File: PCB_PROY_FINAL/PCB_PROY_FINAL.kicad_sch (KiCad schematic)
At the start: 3 parts

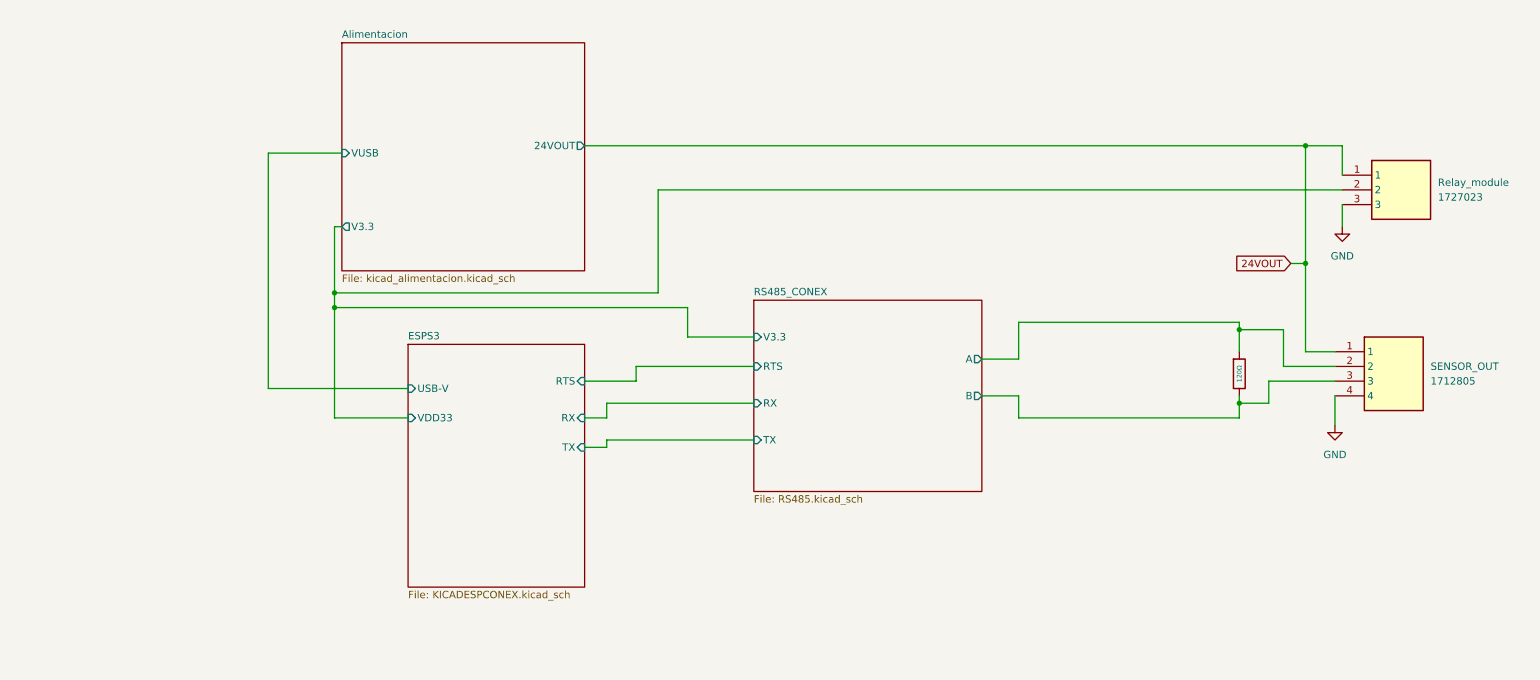
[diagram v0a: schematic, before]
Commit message: Last update pcb
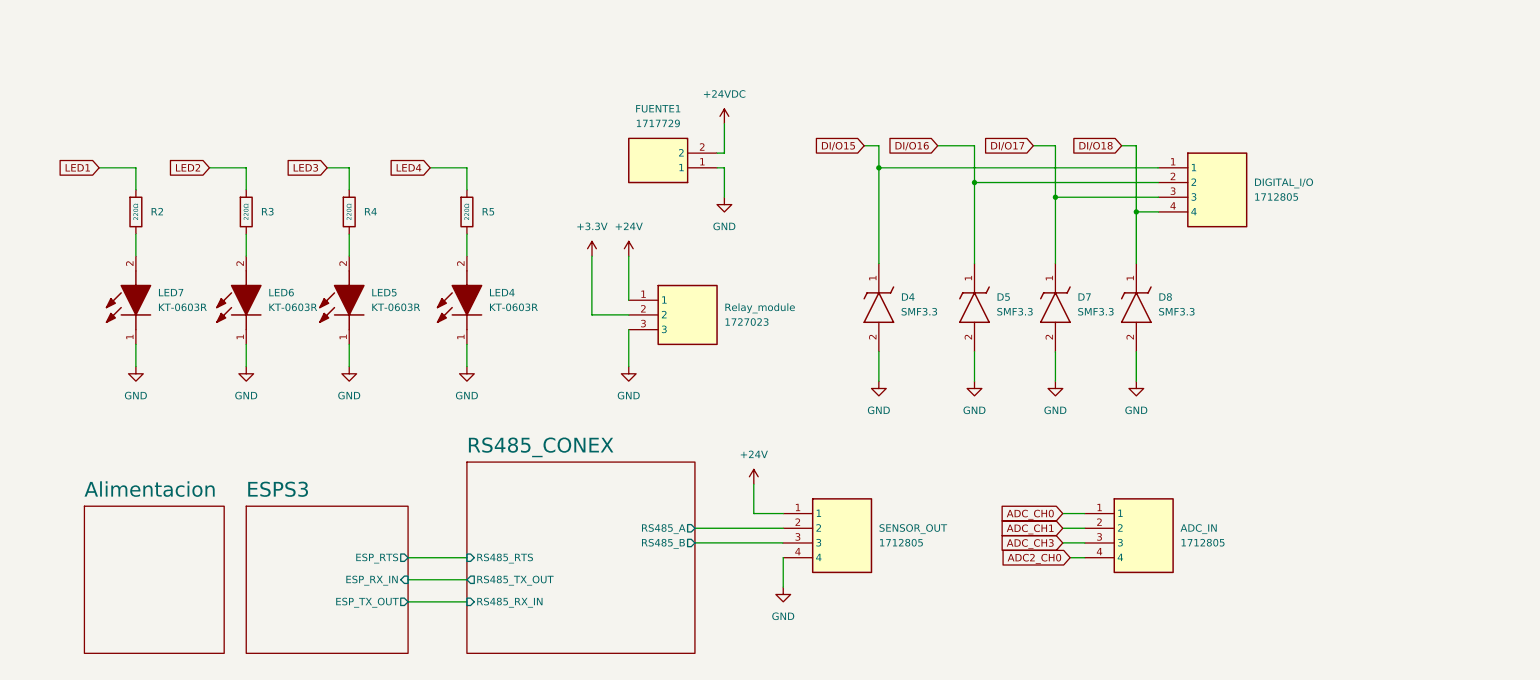
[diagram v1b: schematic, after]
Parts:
- removed R2: 120Ω, PCM_JLCPCB:R_1206, symbol PCM_JLCPCB-Resistors:1206,120Ω
- added ADC_IN, DIGITAL_I/O: 1712805, 1712805, symbol SamacSys_Parts:1712805
- added D4, D5, D7, D8: SMF3.3, SamacSys_Parts:SOD3718X108N, symbol SamacSys_Parts:SMF3.3
- added FUENTE1: 1717729, 1717729, symbol SamacSys_Parts:1717729
- added LED4, LED5, LED6, LED7: KT-0603R, LEDC1608X70N, symbol SamacSys_Parts:KT-0603R
- added R2, R3, R4, R5: 220Ω, PCM_JLCPCB:R_0603, symbol PCM_JLCPCB-Resistors:0603,220Ω
- SENSOR_OUT: JLC PART# (none) -> C90087
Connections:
- net GND: now also D4.2 (A), D5.2 (A), D7.2 (A), D8.2 (A), FUENTE1.1, LED4.1 (K), LED5.1 (K), LED6.1 (K), LED7.1 (K)
- net 24VOUT renamed +24V
- net Alimentacion/V3.3 renamed +3.3V
- net RS485_CONEX/A renamed RS485_CONEX/RS485_A
- net RS485_CONEX/B renamed RS485_CONEX/RS485_B
- new net: LED7.2 (A), R2.2
- new net: LED5.2 (A), R4.2
- new net: LED4.2 (A), R5.2
- new net: LED6.2 (A), R3.2
- new net +24VDC: FUENTE1.2
- new net ADC2_CH0: ADC_IN.4
- new net ADC_CH0: ADC_IN.1
- new net ADC_CH1: ADC_IN.2
- new net ADC_CH3: ADC_IN.3
- new net DI/O15: D4.1 (K), DIGITAL_I/O.1
- new net DI/O16: D5.1 (K), DIGITAL_I/O.2
- new net DI/O17: D7.1 (K), DIGITAL_I/O.3
- new net DI/O18: D8.1 (K), DIGITAL_I/O.4
- new net LED1: R2.1
- new net LED2: R3.1
- new net LED3: R4.1
- new net LED4: R5.1
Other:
- sheet Alimentacion ports: added none; removed 24VOUT, V3.3, VUSB
- sheet ESPS3 ports: added ESP_RTS, ESP_RX_IN, ESP_TX_OUT; removed RTS, RX, TX, USB-V, VDD33
- sheet RS485_CONEX ports: added RS485_A, RS485_B, RS485_RTS, RS485_RX_IN, RS485_TX_OUT; removed A, B, RTS, RX, TX, V3.3
- moved on the sheet: Relay_module, SENSOR_OUT

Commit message: new changes
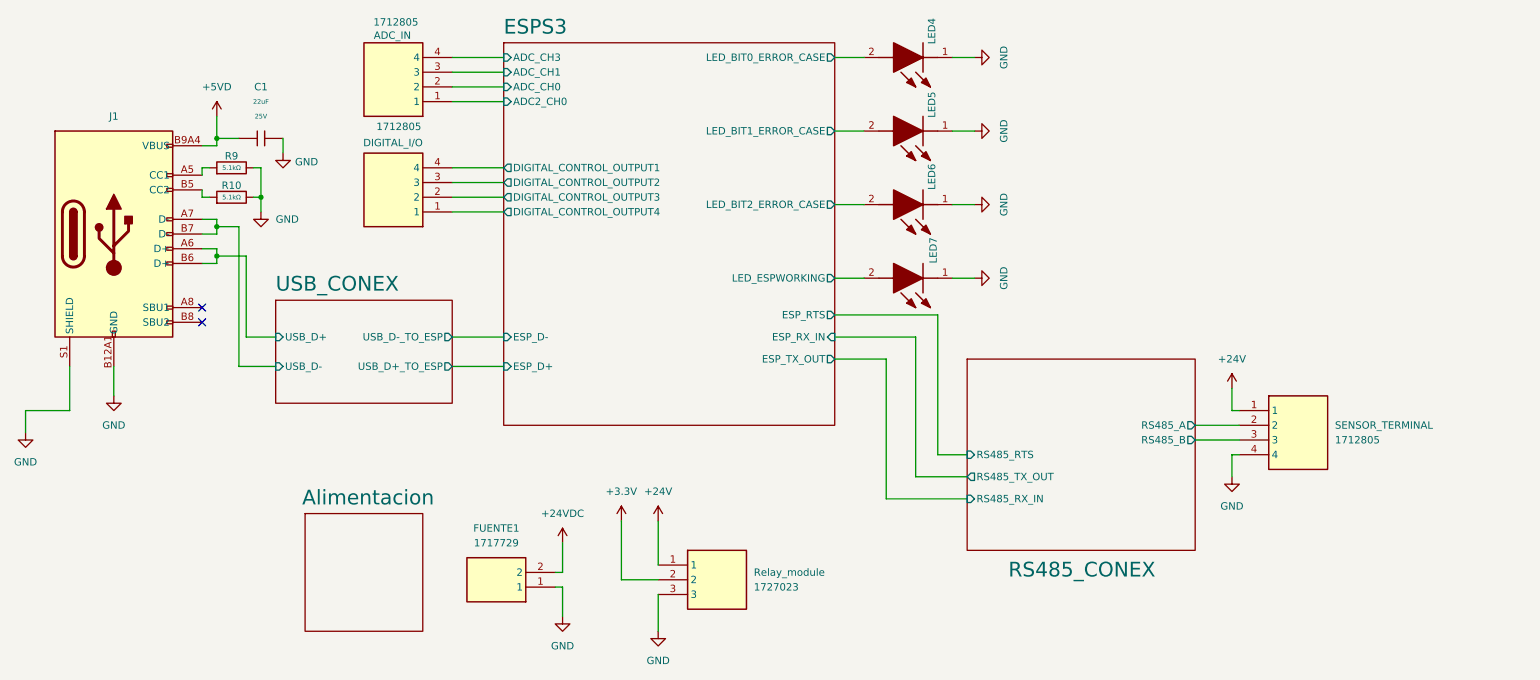
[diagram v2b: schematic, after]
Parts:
- removed D4, D5, D7, D8: SMF3.3, SamacSys_Parts:SOD3718X108N, symbol SamacSys_Parts:SMF3.3
- removed R2, R3, R4, R5: 220Ω, PCM_JLCPCB:R_0603, symbol PCM_JLCPCB-Resistors:0603,220Ω
- added C1: 22uF, PCM_JLCPCB:C_0805, symbol PCM_JLCPCB-Capacitors:0805,22uF
- added J1: Connector, USB-TYPE-C-16P, PCM_JLCPCB:TYPE-C-SMD_HX-TYPE-C-16PIN, symbol PCM_JLCPCB-Extended:Connector, USB-TYPE-C-16P
- added R10, R9: 5.1kΩ, PCM_JLCPCB:R_0805, symbol PCM_JLCPCB-Resistors:0805,5.1kΩ
- renumbered SENSOR_OUT to SENSOR_TERMINAL
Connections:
- net GND: now also C1.2, J1.A12B1 (GND), J1.B12A1 (GND), J1.S1 (SHIELD), R10.2, R9.2
- net ESPS3/LED_ESPWORKING: now reaches LED7.2 (A)
- net ESPS3/LED_BIT1_ERROR_CASE: now reaches LED5.2 (A)
- net ESPS3/LED_BIT0_ERROR_CASE: now reaches LED4.2 (A)
- net ESPS3/LED_BIT2_ERROR_CASE: now reaches LED6.2 (A)
- net ADC2_CH0 renamed ESPS3/ADC_CH3
- net ADC_CH0 renamed ESPS3/ADC2_CH0
- net ADC_CH1 renamed ESPS3/ADC_CH0
- net ADC_CH3 renamed ESPS3/ADC_CH1
- net DI/O15 renamed ESPS3/DIGITAL_CONTROL_OUTPUT4
- net DI/O16 renamed ESPS3/DIGITAL_CONTROL_OUTPUT3
- net DI/O17 renamed ESPS3/DIGITAL_CONTROL_OUTPUT2
- net DI/O18 renamed ESPS3/DIGITAL_CONTROL_OUTPUT1
- new net: J1.A5 (CC1), R9.1
- new net: J1.B5 (CC2), R10.1
- new net +5VD: C1.1, J1.A9B4 (VBUS), J1.B9A4 (VBUS)
- new net USB_CONEX/USB_D+: J1.A6 (D+), J1.B6 (D+)
- new net USB_CONEX/USB_D-: J1.A7 (D-), J1.B7 (D-)
- no-connect marks 0 -> 2
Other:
- added sheet USB_CONEX (USB.kicad_sch)
- sheet ESPS3 ports: added ADC2_CH0, ADC_CH0, ADC_CH1, ADC_CH3, DIGITAL_CONTROL_OUTPUT1, DIGITAL_CONTROL_OUTPUT2, DIGITAL_CONTROL_OUTPUT3, DIGITAL_CONTROL_OUTPUT4, ESP_D+, ESP_D-, LED_BIT0_ERROR_CASE, LED_BIT1_ERROR_CASE, LED_BIT2_ERROR_CASE, LED_ESPWORKING; removed none
- moved on the sheet: ADC_IN, DIGITAL_I/O, FUENTE1, LED4, LED5, LED6, LED7, Relay_module, SENSOR_TERMINAL
